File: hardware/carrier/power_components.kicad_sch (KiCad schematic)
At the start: 38 parts, among them J6 USB4235, J7 BATTERY, Q4 AO3401A, SW2 JS102011SAQN, U5 BQ25185DLHR, U6 MAX17048G+T10, U7 TPS62840DLCR

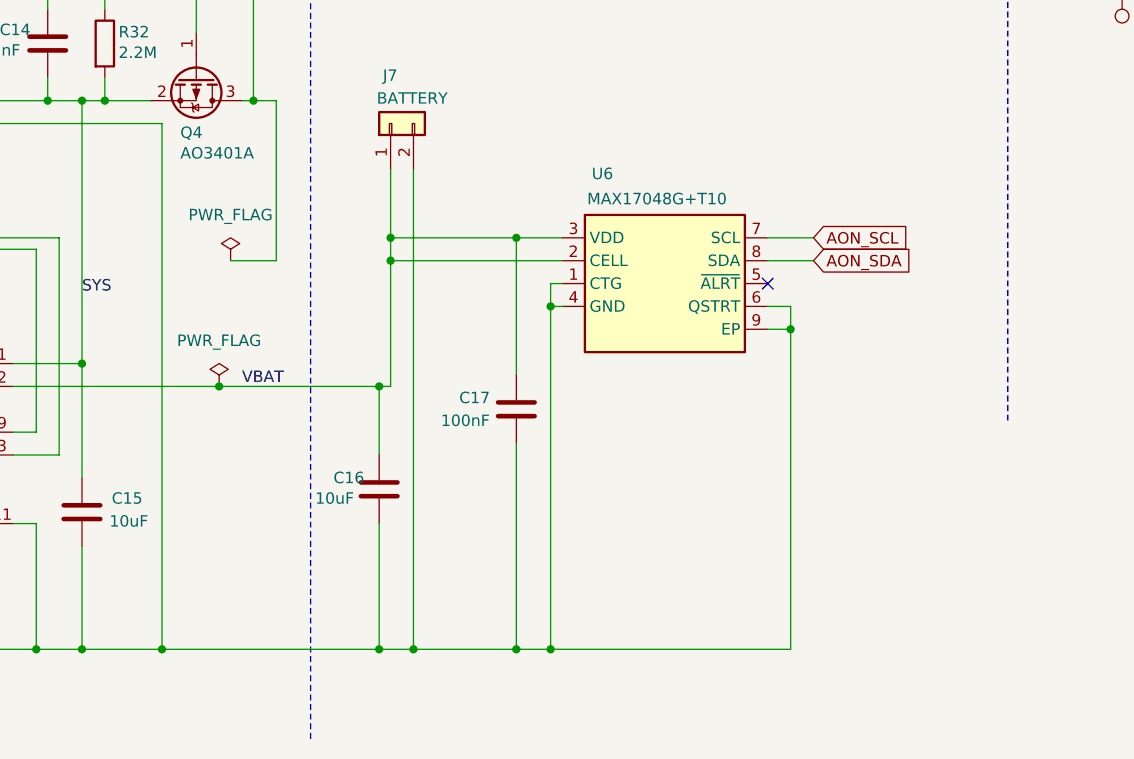
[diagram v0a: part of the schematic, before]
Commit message: Attempt to layout the PCB
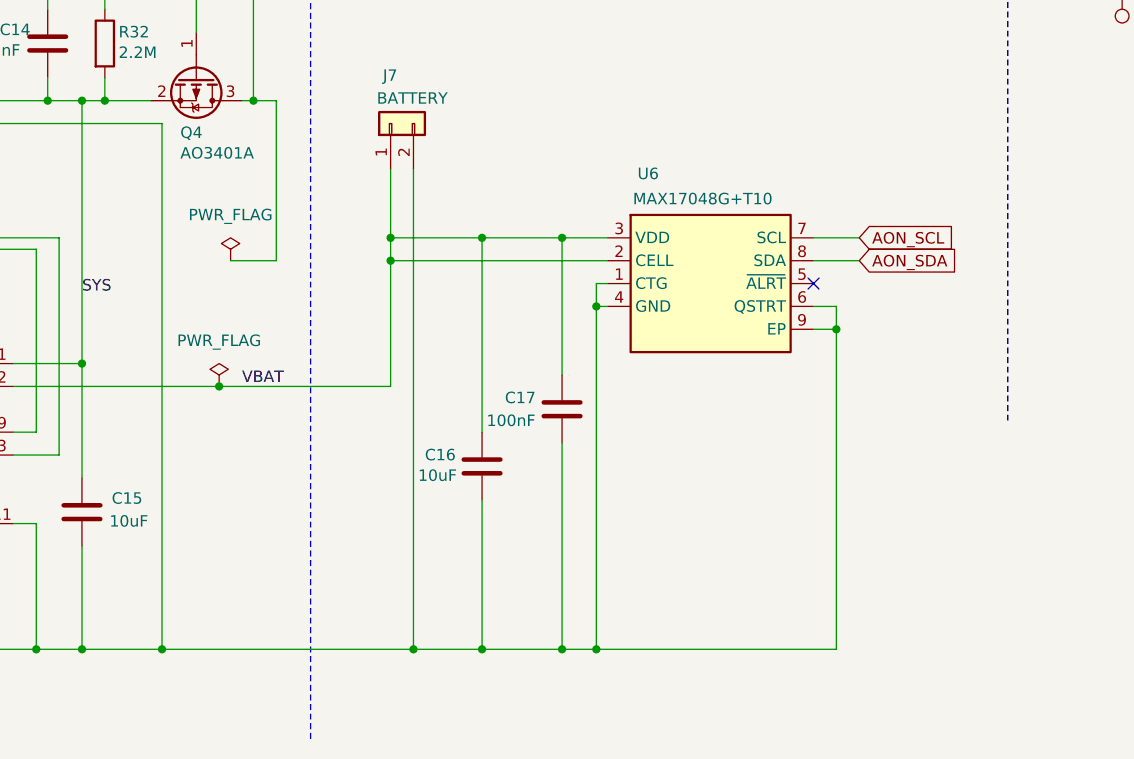
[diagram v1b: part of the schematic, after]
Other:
- moved on the sheet: C16, C17, U6
